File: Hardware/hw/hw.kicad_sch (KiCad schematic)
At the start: 2 parts, among them U1 ESP32-C6-WROOM-1, U2 RV-3028-C7

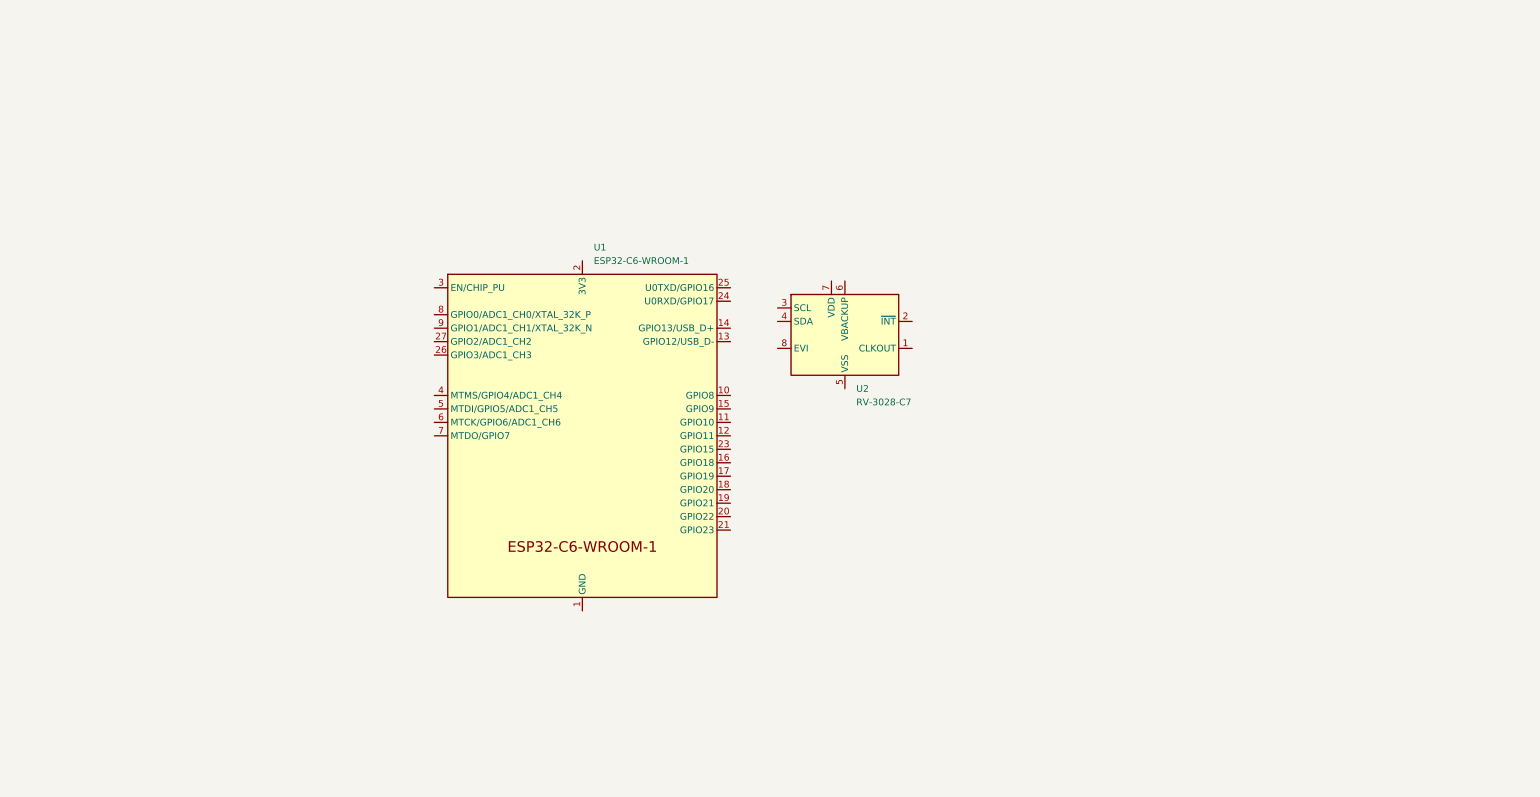
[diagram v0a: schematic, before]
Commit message: Scheme update
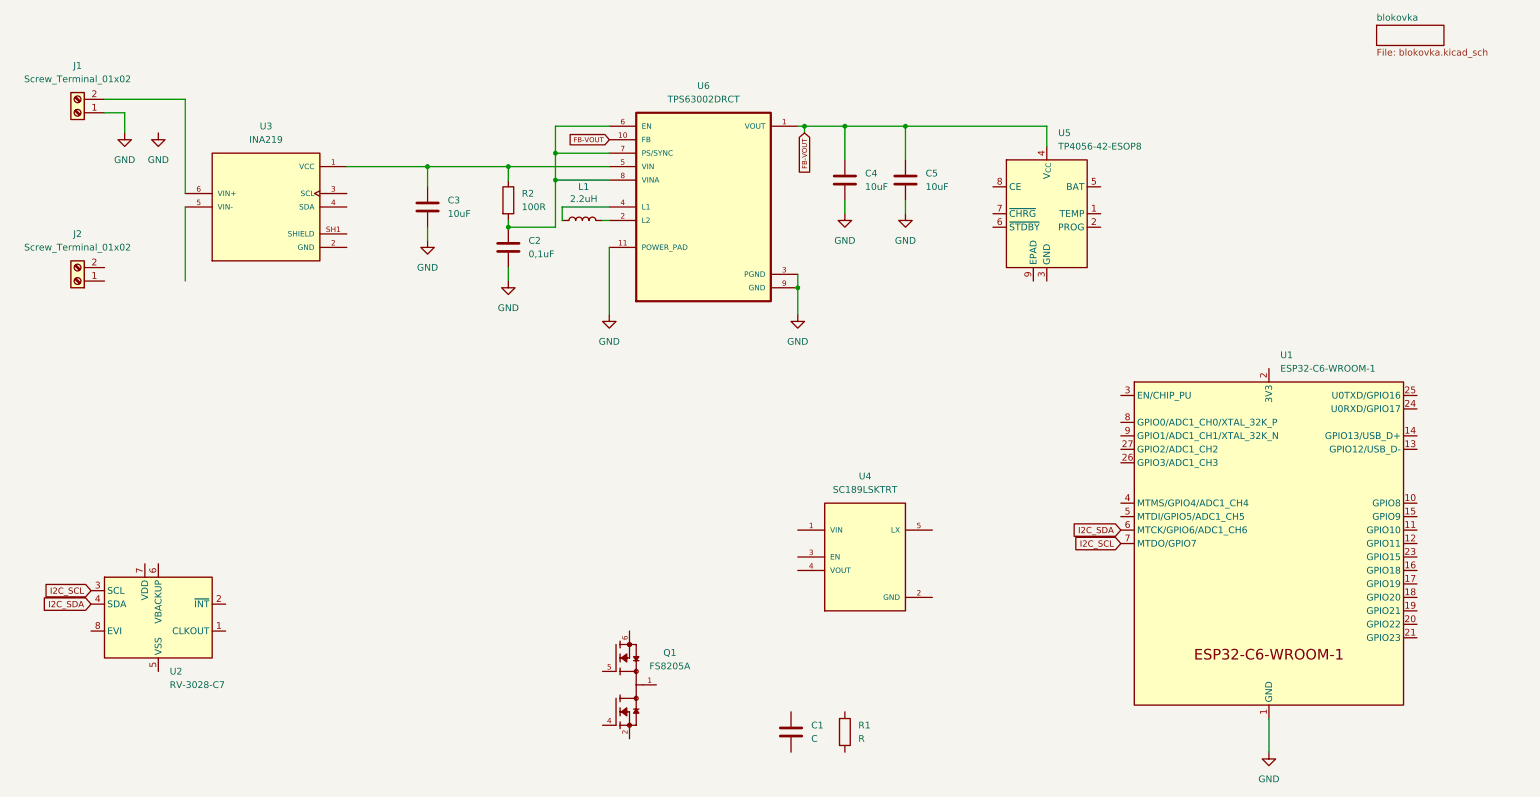
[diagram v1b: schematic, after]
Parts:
- added C1: C, Capacitor_SMD:C_0805_2012Metric, symbol Device:C
- added C2: 0,1uF, Capacitor_SMD:C_0805_2012Metric, symbol Device:C
- added C3, C4, C5: 10uF, Capacitor_SMD:C_0805_2012Metric, symbol Device:C
- added J1, J2: Screw_Terminal_01x02, TerminalBlock_Phoenix:TerminalBlock_Phoenix_MPT-0,5-2-2.54_1x02_P2.54mm_Horizontal, symbol Connector:Screw_Terminal_01x02
- added L1: 2.2uH, Inductor_SMD:L_0201_0603Metric, symbol Device:L
- added Q1: FS8205A, FS8205A:SOP65P640X120-8N, symbol FS8205A:FS8205A
- added R1: R, Resistor_SMD:R_0805_2012Metric, symbol Device:R
- added R2: 100R, Resistor_SMD:R_0805_2012Metric, symbol Device:R
- added U3: INA219, INA219:MODULE_INA219, symbol INA219:INA219
- added U4: SC189LSKTRT, SC189LSKTRT:SOT95P280X145-5N, symbol SC189LSKTRT:SC189LSKTRT
- added U5: TP4056-42-ESOP8, Package_SO:SOIC-8-1EP_3.9x4.9mm_P1.27mm_EP2.41x3.3mm_ThermalVias, symbol Battery_Management:TP4056-42-ESOP8
- added U6: TPS63002DRCT, TPS63002DRCT:VREG_V62_16624-01YE, symbol TPS63002DRCT:TPS63002DRCT
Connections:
- net I2C_SCL: now reaches U2.3 (SCL)
- net I2C_SCL: now also U1.7 (MTDO/GPIO7)
- net I2C_SDA: now reaches U2.4 (SDA)
- net I2C_SDA: now also U1.6 (MTCK/GPIO6/ADC1_CH6)
- net GND: now reaches U1.1 (GND), U1.28 (GND), U1.29 (GND)
- net GND: now also C2.2, C3.2, C4.2, C5.2, J1.1 (Pin_1), U6.11 (POWER_PAD), U6.3 (PGND), U6.9 (GND)
- new net: L1.1, U6.4 (L1)
- new net: L1.2, U6.2 (L2)
- new net: C2.1, R2.2, U6.6 (EN), U6.7 (PS/SYNC), U6.8 (VINA)
- new net: J1.2 (Pin_2), U3.6 (VIN+), U3.VIN+
- new net: C3.1, R2.1, U3.1 (VCC), U6.5 (VIN)
- new net: U3.5 (VIN-), U3.VIN-
- new net: U3.SH1 (SHIELD), U3.SH2 (SHIELD), U3.SH3 (SHIELD), U3.SH4 (SHIELD)
- new net: Q1.1, Q1.8
- new net: Q1.2, Q1.3
- new net: Q1.6, Q1.7
- new net FB-VOUT: C4.1, C5.1, U5.4 (V_{CC}), U6.1 (VOUT), U6.10 (FB)
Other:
- added sheet blokovka (blokovka.kicad_sch)
- moved on the sheet: U1, U2
